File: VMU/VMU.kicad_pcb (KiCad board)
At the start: 4 copper layers, 76.2 x 53.3 mm, 56 parts, among them J1 TBL009-254-14GY-2GY, J15 ARM_JTAG_SWD_10, J16 Conn_01x02_Pin, J2 TBL009-254-14GY-2GY, J3 TBL009-254-14GY-2GY, J4 TBL009-254-14GY-2GY, J7 Conn_01x08_Pin, J8 Conn_01x08_Pin, U1 TLV9064, U2 TLV9064, U3 ADP150AUJZ-3.3-R7, U4 SN65HVD233, U5 STM32F091RCTx

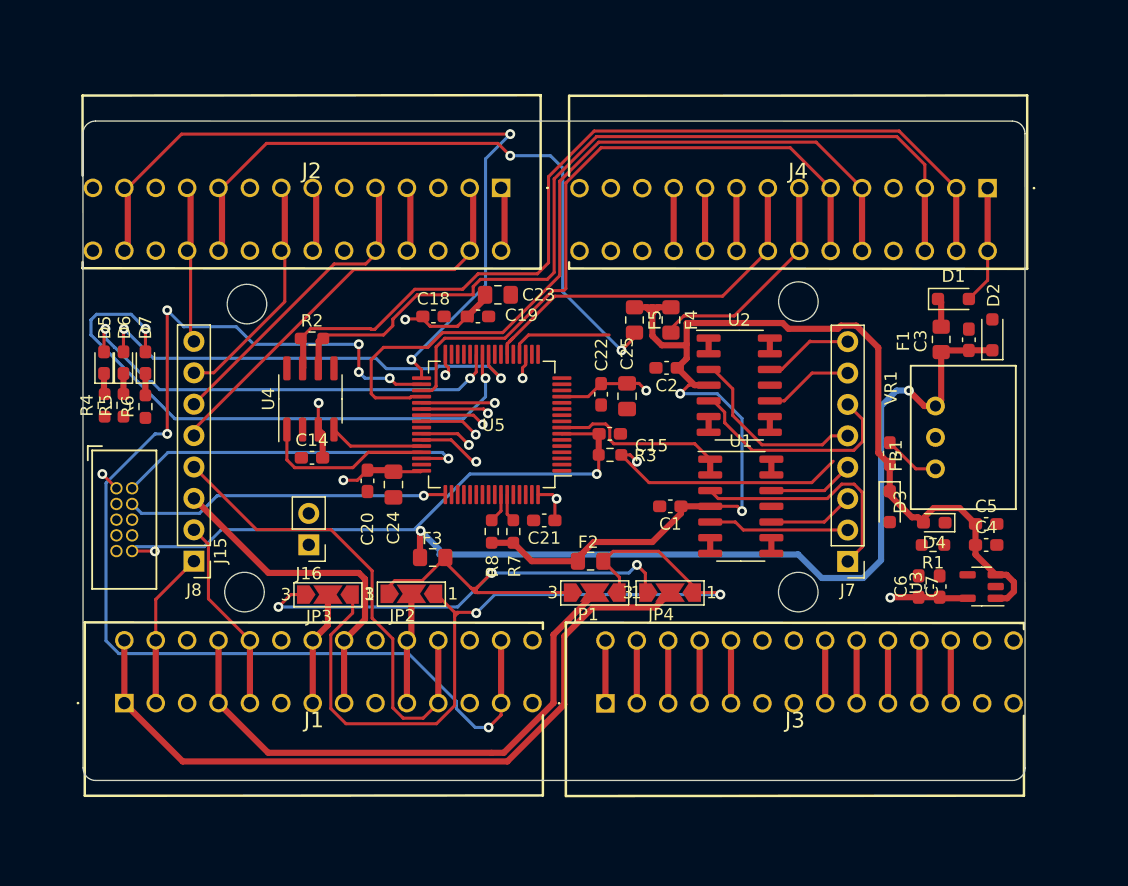
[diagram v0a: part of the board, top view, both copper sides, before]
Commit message: RoutingV2
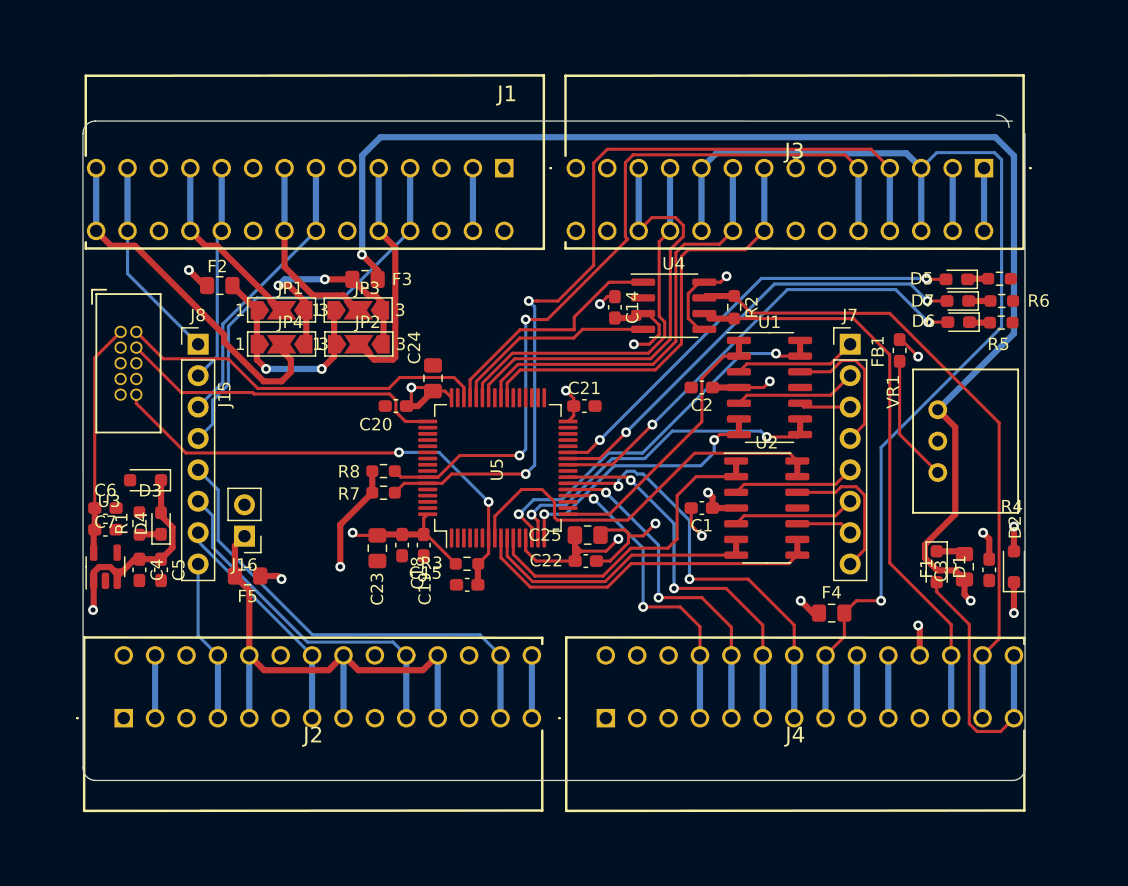
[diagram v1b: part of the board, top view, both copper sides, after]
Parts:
- moved R4 73.1 mm to (165.6, 89.0), turned to 180 degrees
- moved R5 71.3 mm to (165.7, 92.5), turned to 180 degrees
- moved U3 70.9 mm to (93.2, 112.2), turned to 90 degrees
- moved R6 69.8 mm to (165.8, 90.8), turned to 180 degrees
- moved D5 69.3 mm to (162.1, 89.0), turned to 180 degrees
- moved C4 68.5 mm to (96.0, 112.5), turned to -90 degrees
- moved D6 67.6 mm to (162.3, 92.5), turned to 180 degrees
- moved C7 67.6 mm to (93.2, 109.2), turned to 0 degrees
- moved C5 66.9 mm to (97.8, 112.5), turned to -90 degrees
- moved C6 66.1 mm to (93.2, 107.5), turned to 0 degrees
- moved D7 65.9 mm to (162.2, 90.8), turned to 180 degrees
- moved R1 64.2 mm to (96.0, 108.8), turned to 90 degrees
- moved D4 62.6 mm to (97.8, 108.8), turned to 90 degrees
- moved D3 60.2 mm to (96.5, 105.2), turned to 180 degrees
- moved J1 53.1 mm to (125.5, 80.0), turned to 180 degrees
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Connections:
- F4 pad 2: /DIGITAL_SUPPLY_3 -> /DIGITAL_SUPPLY_1
- F5 pad 2: /SUPPLY_8 -> /PB_SUPPLY
- J1 pad 1: /SUPPLY_1 -> GND
- J1 pad 10: /ANALOG_2_SIGNAL -> /SUPPLY_4
- J1 pad 13: /SUPPLY_3 -> /ANALOG_3_SIGNAL
- J1 pad 14: /SUPPLY_3 -> /ANALOG_3_SIGNAL
- J1 pad 15: /ANALOG_3_SIGNAL -> /SUPPLY_3
- J1 pad 16: /ANALOG_3_SIGNAL -> /SUPPLY_3
- J1 pad 19: /SUPPLY_4 -> /ANALOG_2_SIGNAL
- J1 pad 2: /SUPPLY_1 -> GND
- J1 pad 20: /SUPPLY_4 -> /ANALOG_2_SIGNAL
- J1 pad 21: /ANALOG_4_SIGNAL -> /SUPPLY_2
- J1 pad 22: /ANALOG_4_SIGNAL -> /SUPPLY_2
- J1 pad 25: /GPIO_SPLY_2 -> /ANALOG_1_SIGNAL
- J1 pad 26: /GPIO_SPLY_2 -> /ANALOG_1_SIGNAL
- J1 pad 27: GND -> /SUPPLY_1
- J1 pad 28: GND -> /SUPPLY_1
- J1 pad 3: /ANALOG_1_SIGNAL -> /GPIO_SPLY_2
- J1 pad 4: /ANALOG_1_SIGNAL -> /GPIO_SPLY_2
- J1 pad 7: /SUPPLY_2 -> /ANALOG_4_SIGNAL
- J1 pad 8: /SUPPLY_2 -> /ANALOG_4_SIGNAL
- J1 pad 9: /ANALOG_2_SIGNAL -> /SUPPLY_4
- J2 pad 1: /SUPPLY_5 -> GND
- J2 pad 10: /ANALOG_6_SIGNAL -> /PB_SUPPLY
- J2 pad 13: /SUPPLY_7 -> /ANALOG_7_SIGNAL
- J2 pad 14: /SUPPLY_7 -> /ANALOG_7_SIGNAL
- J2 pad 15: /ANALOG_7_SIGNAL -> /PB_SUPPLY
- J2 pad 16: /ANALOG_7_SIGNAL -> /PB_SUPPLY
- J2 pad 19: /SUPPLY_8 -> /ANALOG_6_SIGNAL
- J2 pad 2: /SUPPLY_5 -> GND
- J2 pad 20: /SUPPLY_8 -> /ANALOG_6_SIGNAL
- J2 pad 21: /ANALOG_8_SIGNAL -> /PB_SUPPLY
- J2 pad 22: /ANALOG_8_SIGNAL -> /PB_SUPPLY
- J2 pad 25: /GPIO_SPLY_1 -> /ANALOG_5_SIGNAL
- J2 pad 26: /GPIO_SPLY_1 -> /ANALOG_5_SIGNAL
- J2 pad 27: GND -> /PB_SUPPLY
- J2 pad 28: GND -> /PB_SUPPLY
- J2 pad 3: /ANALOG_5_SIGNAL -> /GPIO_SPLY_1
- J2 pad 4: /ANALOG_5_SIGNAL -> /GPIO_SPLY_1
- J2 pad 7: /SUPPLY_6 -> /ANALOG_8_SIGNAL
- J2 pad 8: /SUPPLY_6 -> /ANALOG_8_SIGNAL
- J2 pad 9: /ANALOG_6_SIGNAL -> /PB_SUPPLY
- J3 pad 19: /DIGITAL_SUPPLY_2 -> /DIGITAL_SUPPLY_1
- J3 pad 20: /DIGITAL_SUPPLY_2 -> /DIGITAL_SUPPLY_1
- J4 pad 1: /battery_in -> GND
- J4 pad 10: /GPIO_SPLY_4 -> /SPI_SCLK
- J4 pad 11: /GPIO_SPLY_3 -> /SPI_MOSI
- J4 pad 12: /GPIO_SPLY_3 -> /SPI_MOSI
- J4 pad 13: /DIGITAL_SUPPLY_3 -> /SPI_MISO
- J4 pad 14: /DIGITAL_SUPPLY_3 -> /SPI_MISO
- J4 pad 15: /SPI_MISO -> /DIGITAL_SUPPLY_1
- J4 pad 16: /SPI_MISO -> /DIGITAL_SUPPLY_1
- J4 pad 17: /SPI_MOSI -> /GPIO_SPLY_3
- J4 pad 18: /SPI_MOSI -> /GPIO_SPLY_3
- J4 pad 19: /SPI_SCLK -> /GPIO_SPLY_4
- J4 pad 2: /battery_in -> GND
- J4 pad 20: /SPI_SCLK -> /GPIO_SPLY_4
- J4 pad 21: /SPI_~{CS} -> GND
- J4 pad 22: /SPI_~{CS} -> GND
- J4 pad 23: GND -> /CAN1_L
- J4 pad 24: GND -> /CAN1_L
- J4 pad 25: GND -> /CAN1_H
- J4 pad 26: GND -> /CAN1_H
- J4 pad 27: GND -> /battery_in
- J4 pad 28: GND -> /battery_in
- J4 pad 3: /CAN1_H -> GND
- J4 pad 4: /CAN1_H -> GND
- J4 pad 5: /CAN1_L -> GND
- J4 pad 6: /CAN1_L -> GND
- J4 pad 7: GND -> /SPI_~{CS}
- J4 pad 8: GND -> /SPI_~{CS}
- J4 pad 9: /GPIO_SPLY_4 -> /SPI_SCLK
- U5 pad 10: /MCU/ANALOG_3 -> /MCU/ANALOG_6
- U5 pad 11: /MCU/ANALOG_4 -> /MCU/ANALOG_5
- U5 pad 14: /MCU/ANALOG_5 -> /MCU/ANALOG_4
- U5 pad 15: /MCU/ANALOG_6 -> /MCU/ANALOG_3
- U5 pad 16: /MCU/ANALOG_7 -> /MCU/ANALOG_2
- U5 pad 17: /MCU/ANALOG_8 -> /MCU/ANALOG_1
- U5 pad 8: /MCU/ANALOG_1 -> /MCU/ANALOG_8
- U5 pad 9: /MCU/ANALOG_2 -> /MCU/ANALOG_7
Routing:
- net /GPIO_SPLY_2: track 95.4 -> 5.08 mm, vias 6 -> 0
- net /DIGITAL_SUPPLY_1: track 5.08 -> 88.4 mm, vias 0 -> 1
- net /I2C_SDA: track 7.36 -> 70.6 mm, vias 0 -> 2
- net /GPIO_SPLY_4: track 65.1 -> 5.08 mm
- net +5V: track 101.9 -> 43.0 mm, vias 2 -> 8
- net /I2C_SCL: track 7.47 -> 64.1 mm, vias 0 -> 2
- net /GPIO_SPLY_1: track 61.2 -> 5.08 mm, vias 2 -> 0
- net /SUPPLY_8: track 53.6 -> 0.00 mm, vias 2 -> 0
- net Net-(JP1-A): track 67.9 -> 17.6 mm
- net /GPIO_SPLY_3: track 54.5 -> 5.08 mm
- net /PB_SUPPLY: track 0.00 -> 48.0 mm
- net +24V: track 68.1 -> 109.6 mm, vias 2 -> 3
- net Net-(JP1-B): track 56.1 -> 19.0 mm, vias 3 -> 2
- net /MCU/ANALOG_8: track 1.27 -> 32.7 mm
- net /SUPPLY_1: track 60.1 -> 29.1 mm
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- added copper zone on In2.Cu, net +5V
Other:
- board size 76.2 x 53.3 mm -> 76.2 x 53.8 mm
